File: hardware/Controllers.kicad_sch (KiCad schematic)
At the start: 1 part

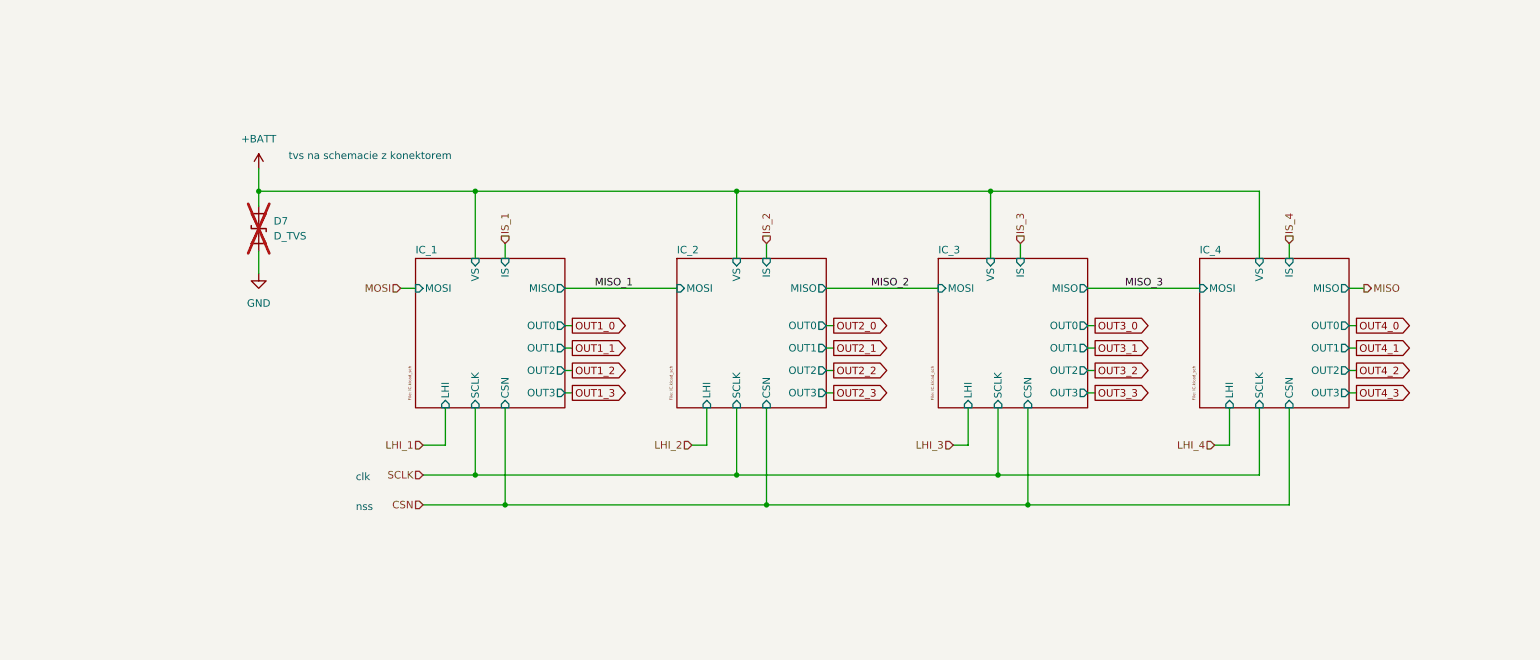
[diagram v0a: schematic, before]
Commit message: NEW SCHEMATIC
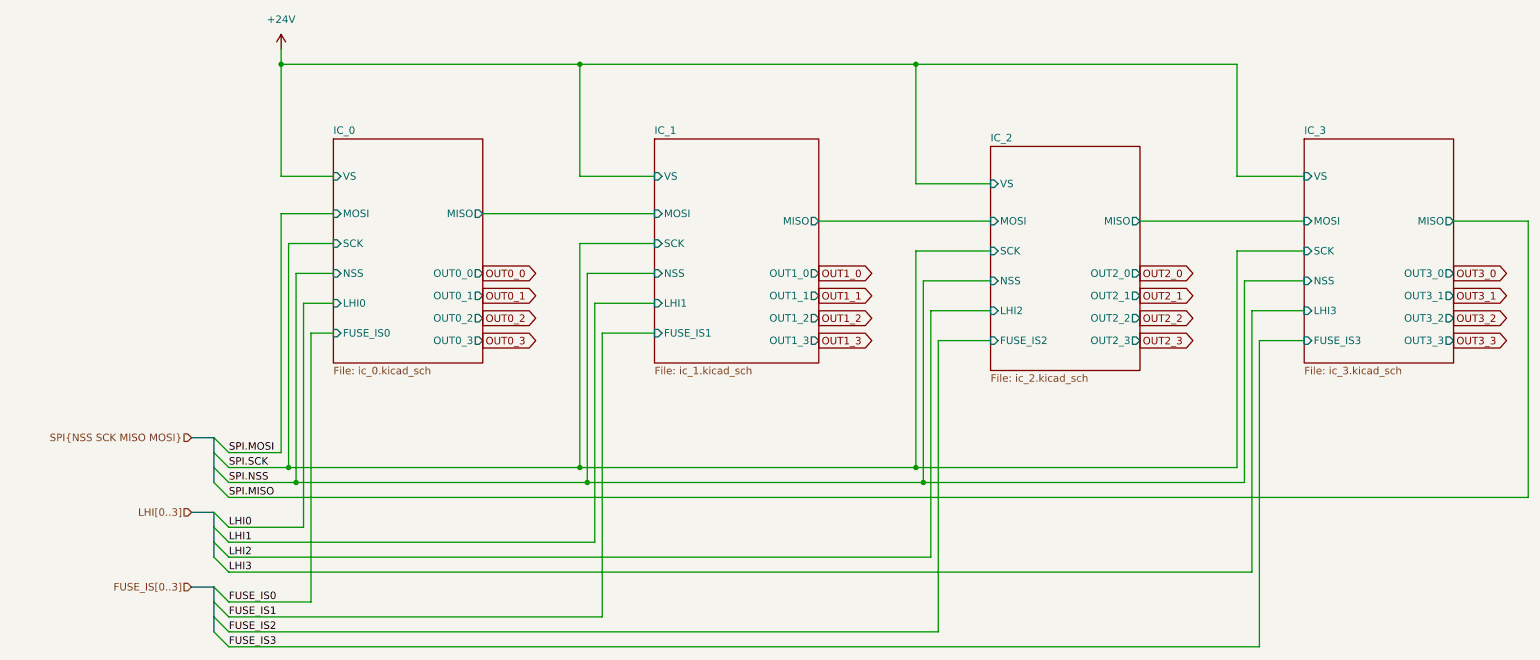
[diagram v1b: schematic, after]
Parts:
- removed D7: D_TVS, symbol Device:D_TVS
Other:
- removed sheet IC_4
- added sheet IC_0 (ic_0.kicad_sch)
- sheet IC_1: file IC.kicad_sch -> ic_1.kicad_sch
- sheet IC_1 ports: added FUSE_IS1, LHI1, NSS, OUT1_0, OUT1_1, OUT1_2, OUT1_3, SCK; removed CSN, IS, LHI, OUT0, OUT1, OUT2, OUT3, SCLK
- sheet IC_2: file IC.kicad_sch -> ic_2.kicad_sch
- sheet IC_2 ports: added FUSE_IS2, LHI2, NSS, OUT2_0, OUT2_1, OUT2_2, OUT2_3, SCK; removed CSN, IS, LHI, OUT0, OUT1, OUT2, OUT3, SCLK
- sheet IC_3: file IC.kicad_sch -> ic_3.kicad_sch
- sheet IC_3 ports: added FUSE_IS3, LHI3, NSS, OUT3_0, OUT3_1, OUT3_2, OUT3_3, SCK; removed CSN, IS, LHI, OUT0, OUT1, OUT2, OUT3, SCLK
- note removed: "clk"
- note removed: "nss"
- note removed: "tvs na schemacie z konektorem"
- company: (none) -> Authors: Grzegorz Potocki Jędrzej Kasprzyk
- title: (none) -> PDUv3
